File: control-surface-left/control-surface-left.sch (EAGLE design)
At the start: 92 parts, among them IC1 74HC595D, IC2 74HC595D, IC3 74HC595D, IC4 74HC595D

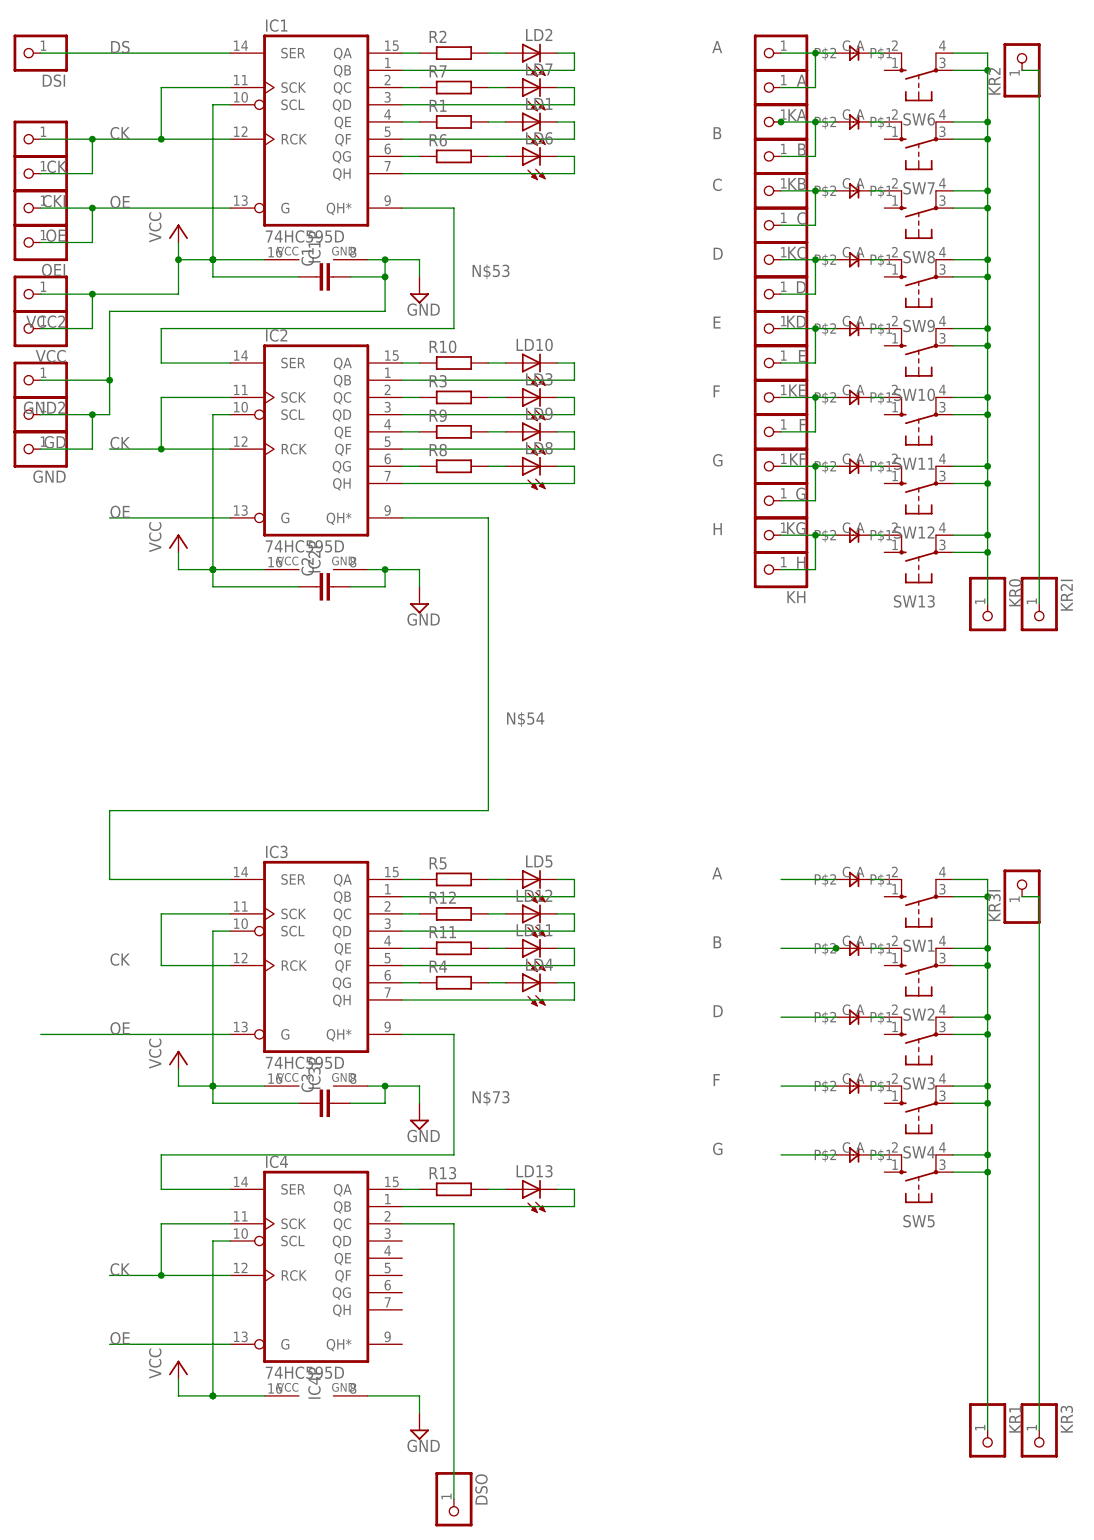
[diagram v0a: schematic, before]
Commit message: mods
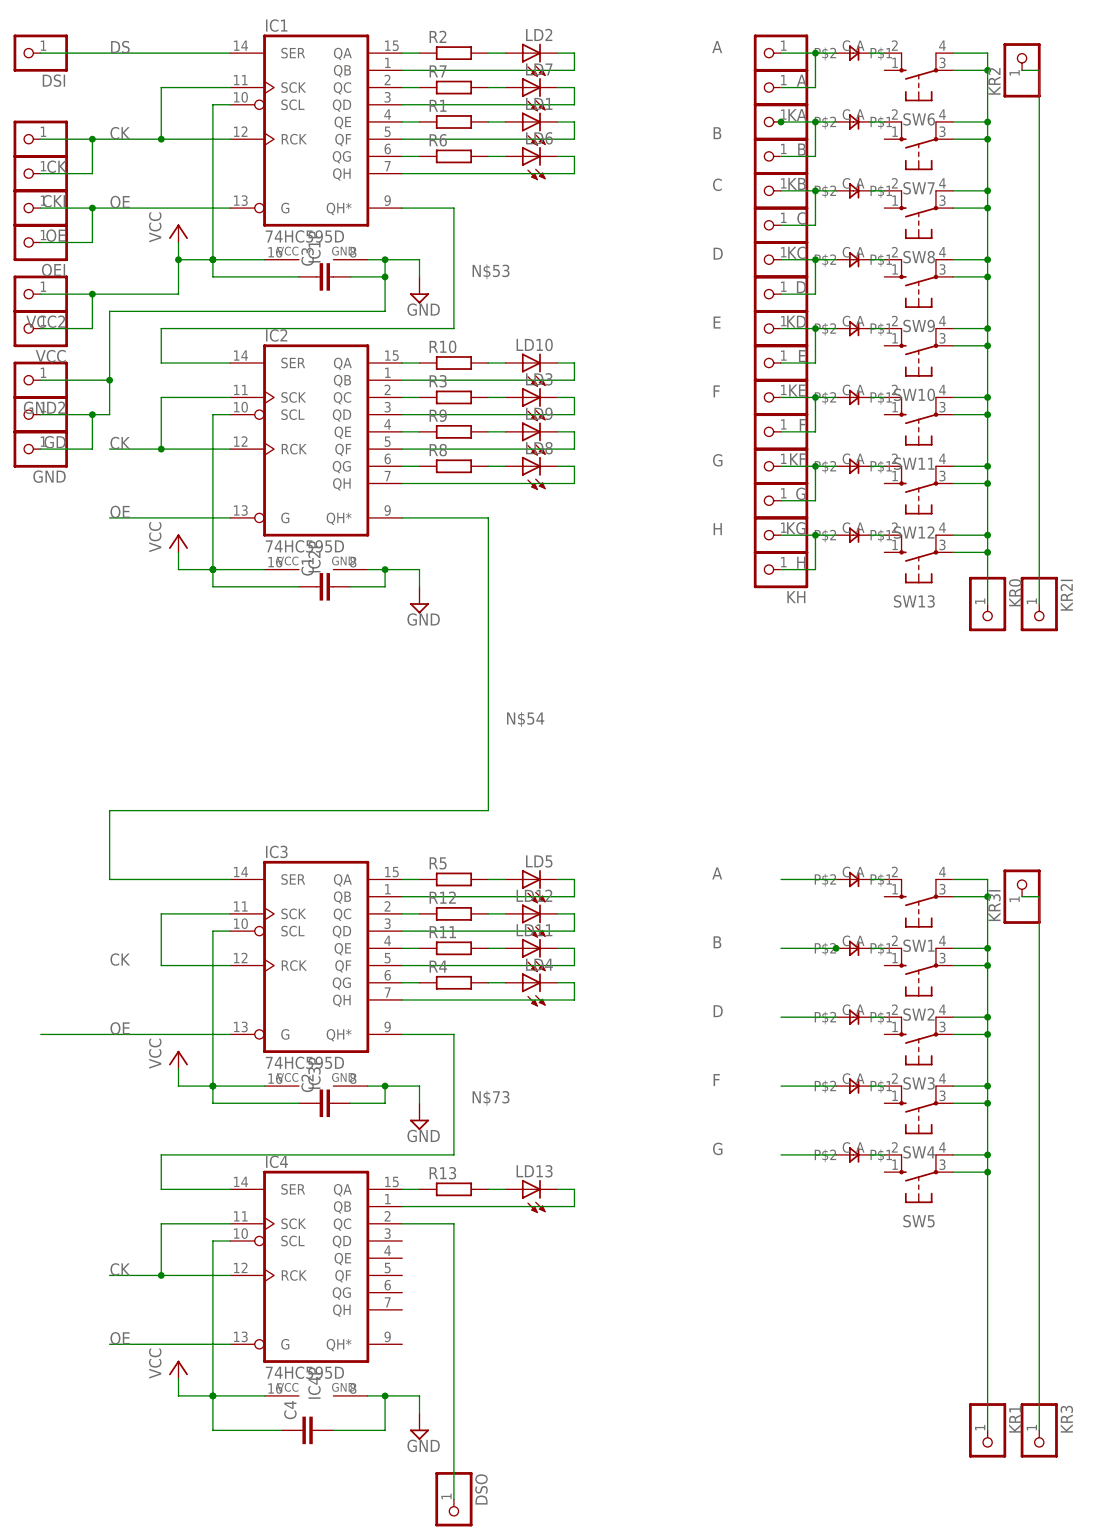
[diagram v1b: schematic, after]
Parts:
- added C4: (no value), rcl:C-EUC0805
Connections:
- net GND: now also C4.2
- net VCC: now also C4.1
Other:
- moved on the sheet: C1, C2, C3
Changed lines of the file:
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@@
 <part name="LD1" library="led" deviceset="LED" device="3MM"/>
 <part name="LD6" library="led" deviceset="LED" device="3MM"/>
-<part name="C1" library="rcl" deviceset="C-EU" device="C0805"/>
+<part name="C3" library="rcl" deviceset="C-EU" device="C0805"/>
 <part name="SUPPLY1" library="supply2" deviceset="GND" device=""/>
 <part name="P+1" library="supply1" deviceset="VCC" device=""/>
@@
 <part name="LD9" library="led" deviceset="LED" device="3MM"/>
 <part name="LD8" library="led" deviceset="LED" device="3MM"/>
-<part name="C2" library="rcl" deviceset="C-EU" device="C0805"/>
+<part name="C1" library="rcl" deviceset="C-EU" device="C0805"/>
 <part name="SUPPLY2" library="supply2" deviceset="GND" device=""/>
 <part name="P+2" library="supply1" deviceset="VCC" device=""/>
@@
 <part name="LD11" library="led" deviceset="LED" device="3MM"/>
 <part name="LD4" library="led" deviceset="LED" device="3MM"/>
-<part name="C3" library="rcl" deviceset="C-EU" device="C0805"/>
+<part name="C2" library="rcl" deviceset="C-EU" device="C0805"/>
 <part name="SUPPLY3" library="supply2" deviceset="GND" device=""/>
 <part name="P+3" library="supply1" deviceset="VCC" device=""/>
@@
 <part name="KH" library="pinhead" deviceset="PINHD-1X1" device=""/>
 <part name="GND" library="pinhead" deviceset="PINHD-1X1" device=""/>
+<part name="C4" library="rcl" deviceset="C-EU" device="C0805"/>
 </parts>
 <sheets>
@@
 <instance part="LD6" gate="G$1" x="73.66" y="45.72" rot="R90"/>
 <instance part="IC1" gate="P" x="43.18" y="30.48" rot="R90"/>
-<instance part="C1" gate="G$1" x="43.18" y="27.94" rot="R90"/>
+<instance part="C3" gate="G$1" x="43.18" y="27.94" rot="R90"/>
 <instance part="SUPPLY1" gate="GND" x="58.42" y="25.4"/>
 <instance part="P+1" gate="VCC" x="22.86" y="35.56"/>
@@
 <instance part="LD8" gate="G$1" x="73.66" y="0" rot="R90"/>
 <instance part="IC2" gate="P" x="43.18" y="-15.24" rot="R90"/>
-<instance part="C2" gate="G$1" x="43.18" y="-17.78" rot="R90"/>
+<instance part="C1" gate="G$1" x="43.18" y="-17.78" rot="R90"/>
 <instance part="SUPPLY2" gate="GND" x="58.42" y="-20.32"/>
 <instance part="P+2" gate="VCC" x="22.86" y="-10.16"/>
@@
 <instance part="LD4" gate="G$1" x="73.66" y="-76.2" rot="R90"/>
 <instance part="IC3" gate="P" x="43.18" y="-91.44" rot="R90"/>
-<instance part="C3" gate="G$1" x="43.18" y="-93.98" rot="R90"/>
+<instance part="C2" gate="G$1" x="43.18" y="-93.98" rot="R90"/>
 <instance part="SUPPLY3" gate="GND" x="58.42" y="-96.52"/>
 <instance part="P+3" gate="VCC" x="22.86" y="-86.36"/>
@@
 <instance part="KH" gate="G$1" x="109.22" y="-15.24" rot="R180"/>
 <instance part="GND" gate="G$1" x="0" y="2.54" rot="R180"/>
+<instance part="C4" gate="G$1" x="40.64" y="-142.24" rot="R90"/>
 </instances>
 <busses>
@@
 <net name="VCC" class="0">
 <segment>
-<pinref part="C1" gate="G$1" pin="1"/>
+<pinref part="C3" gate="G$1" pin="1"/>
 <wire x1="40.64" y1="27.94" x2="27.94" y2="27.94" width="0.1524" layer="91"/>
 <wire x1="27.94" y1="27.94" x2="27.94" y2="30.48" width="0.1524" layer="91"/>
@@
 </segment>
 <segment>
-<pinref part="C2" gate="G$1" pin="1"/>
+<pinref part="C1" gate="G$1" pin="1"/>
 <wire x1="40.64" y1="-17.78" x2="27.94" y2="-17.78" width="0.1524" layer="91"/>
 <wire x1="27.94" y1="-17.78" x2="27.94" y2="-15.24" width="0.1524" layer="91"/>
@@
 </segment>
 <segment>
-<pinref part="C3" gate="G$1" pin="1"/>
+<pinref part="C2" gate="G$1" pin="1"/>
 <wire x1="40.64" y1="-93.98" x2="27.94" y2="-93.98" width="0.1524" layer="91"/>
 <wire x1="27.94" y1="-93.98" x2="27.94" y2="-91.44" width="0.1524" layer="91"/>
@@
 <wire x1="27.94" y1="-114.3" x2="27.94" y2="-137.16" width="0.1524" layer="91"/>
 <junction x="27.94" y="-137.16"/>
+<pinref part="C4" gate="G$1" pin="1"/>
+<wire x1="38.1" y1="-142.24" x2="27.94" y2="-142.24" width="0.1524" layer="91"/>
+<wire x1="27.94" y1="-142.24" x2="27.94" y2="-137.16" width="0.1524" layer="91"/>
 </segment>
 </net>
 <net name="GND" class="0">
 <segment>
-<pinref part="C1" gate="G$1" pin="2"/>
+<pinref part="C3" gate="G$1" pin="2"/>
 <wire x1="48.26" y1="27.94" x2="53.34" y2="27.94" width="0.1524" layer="91"/>
 <wire x1="53.34" y1="27.94" x2="53.34" y2="30.48" width="0.1524" layer="91"/>
@@
 </segment>
 <segment>
-<pinref part="C2" gate="G$1" pin="2"/>
+<pinref part="C1" gate="G$1" pin="2"/>
 <wire x1="48.26" y1="-17.78" x2="53.34" y2="-17.78" width="0.1524" layer="91"/>
 <wire x1="53.34" y1="-17.78" x2="53.34" y2="-15.24" width="0.1524" layer="91"/>
@@
 </segment>
 <segment>
-<pinref part="C3" gate="G$1" pin="2"/>
+<pinref part="C2" gate="G$1" pin="2"/>
 <wire x1="48.26" y1="-93.98" x2="53.34" y2="-93.98" width="0.1524" layer="91"/>
 <wire x1="53.34" y1="-93.98" x2="53.34" y2="-91.44" width="0.1524" layer="91"/>
@@
 <pinref part="IC4" gate="P" pin="GND"/>
 <pinref part="SUPPLY4" gate="GND" pin="GND"/>
-<wire x1="50.8" y1="-137.16" x2="58.42" y2="-137.16" width="0.1524" layer="91"/>
+<wire x1="50.8" y1="-137.16" x2="53.34" y2="-137.16" width="0.1524" layer="91"/>
+<wire x1="53.34" y1="-137.16" x2="58.42" y2="-137.16" width="0.1524" layer="91"/>
 <wire x1="58.42" y1="-137.16" x2="58.42" y2="-139.7" width="0.1524" layer="91"/>
-</segment>
-</net>
+<pinref part="C4" gate="G$1" pin="2"/>
+<wire x1="45.72" y1="-142.24" x2="53.34" y2="-142.24" width="0.1524" layer="91"/>
+<wire x1="53.34" y1="-142.24" x2="53.34" y2="-137.16" width="0.1524" layer="91"/>
+<junction x="53.34" y="-137.16"/>
+</segment>
+</net>
